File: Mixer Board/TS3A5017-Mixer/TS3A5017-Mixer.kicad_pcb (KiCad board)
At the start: 2 copper layers, 6 parts, among them J1 Conn_Coaxial_Small, J2 Conn_Coaxial_Small, J3 Conn_Coaxial_Small, U1 TS3A5017RGY, U2 LMP7715MF

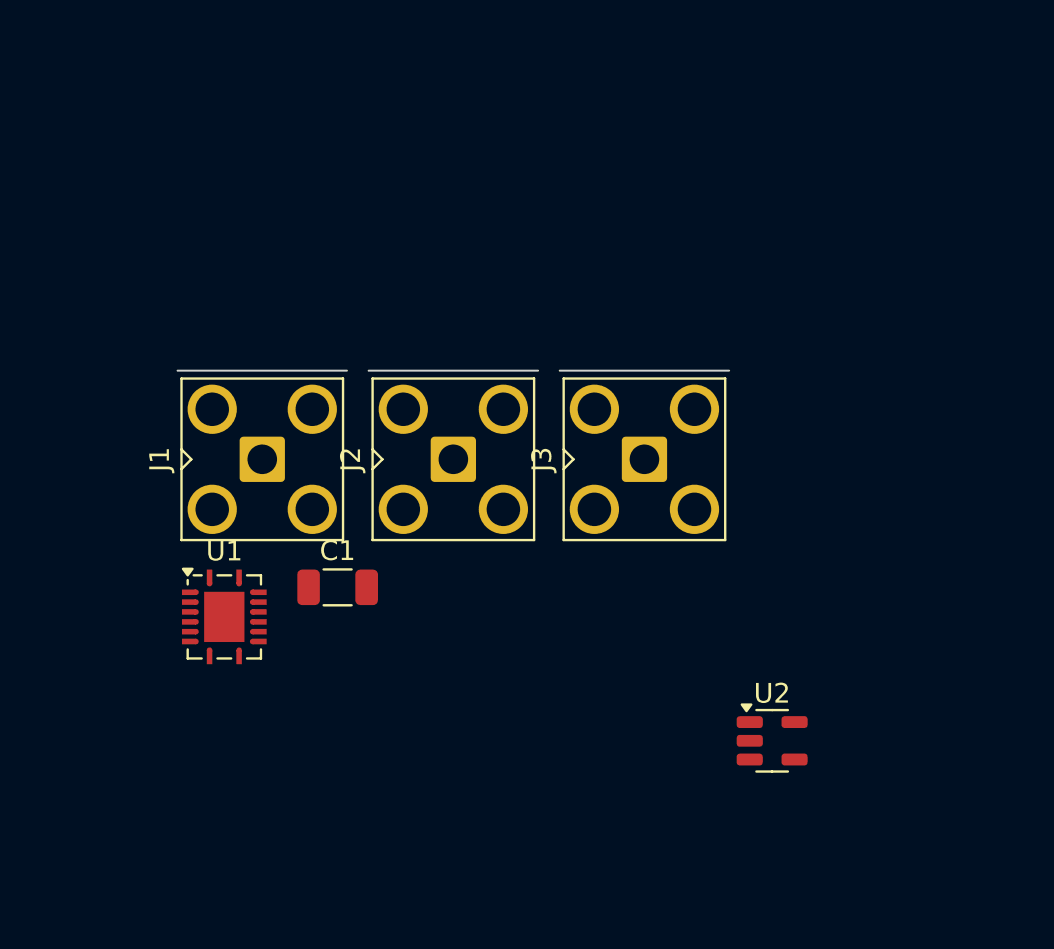
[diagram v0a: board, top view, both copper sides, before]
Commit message: Continued work and first iteration
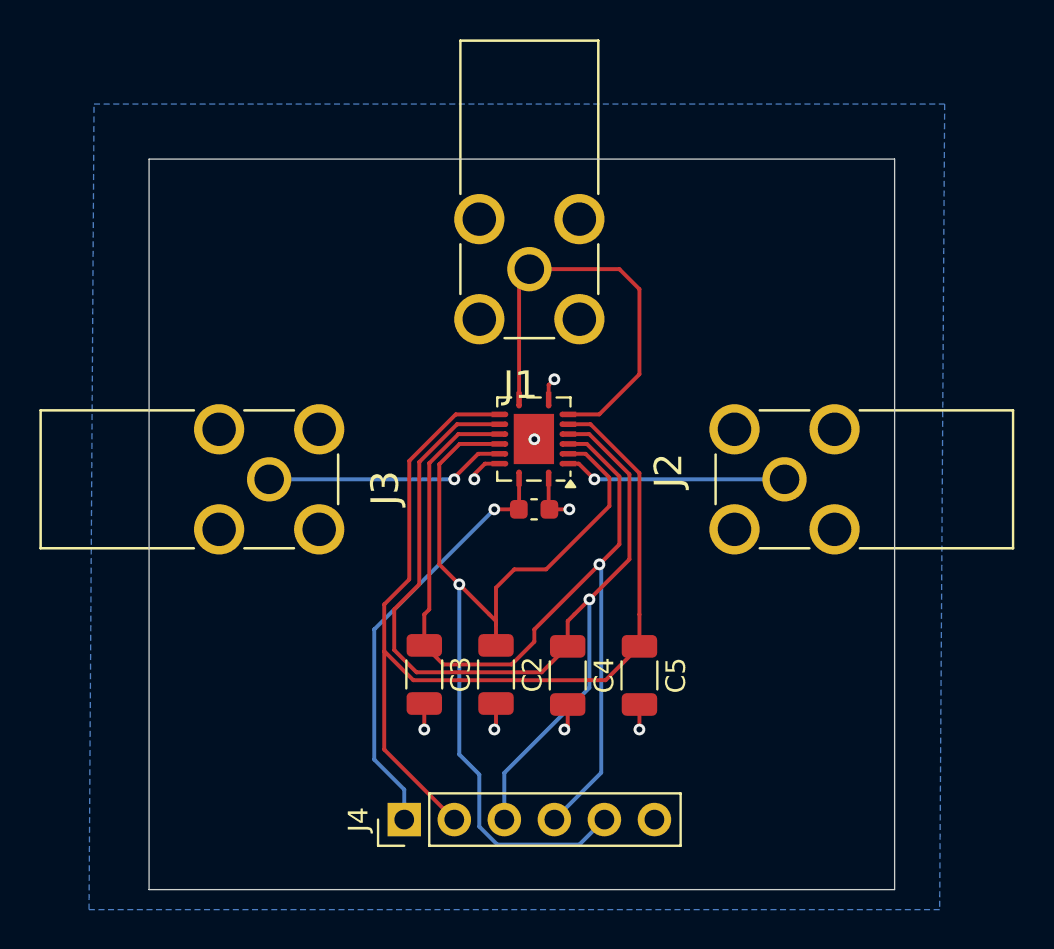
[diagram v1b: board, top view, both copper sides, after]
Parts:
- removed U2: LMP7715MF, Package_TO_SOT_SMD:SOT-23-5
- added C2: .1uf, Capacitor_SMD:C_1206_3216Metric, F.Cu at (144.9, 99.8)
- added C3: .1uf, Capacitor_SMD:C_1206_3216Metric, F.Cu at (141.2, 99.8)
- added C4: .1uf, Capacitor_SMD:C_1206_3216Metric, F.Cu at (148.5, 99.9)
- added C5: .1uf, Capacitor_SMD:C_1206_3216Metric, F.Cu at (152.1, 99.9)
- added J4: Conn_01x06, Connector_PinHeader_2.54mm:PinHeader_1x06_P2.54mm_Vertical, F.Cu at (140.2, 107.2)
- C1: footprint Capacitor_SMD:C_1206_3216Metric -> Capacitor_SMD:C_0603_1608Metric
- J1: value Conn_Coaxial_Small -> RF-In; footprint Connector_Coaxial:SMA_Amphenol_901-143_Horizontal -> Connector_Amphenol:AMPHENOL_901-143-6RFX
- J2: value Conn_Coaxial_Small -> CLK0; footprint Connector_Coaxial:SMA_Amphenol_901-143_Horizontal -> Connector_Amphenol:AMPHENOL_901-143-6RFX
- J3: value Conn_Coaxial_Small -> CLK1; footprint Connector_Coaxial:SMA_Amphenol_901-143_Horizontal -> Connector_Amphenol:AMPHENOL_901-143-6RFX
- moved J3 19.1 mm to (133.3, 89.9), turned to -90 degrees
- moved U1 18.1 mm to (146.8, 87.9), turned to 180 degrees
- moved J2 16.8 mm to (159.5, 89.9), turned to 90 degrees
- moved J1 16.6 mm to (146.6, 79.2), turned to 180 degrees
- moved C1 10.7 mm to (146.8, 91.4)
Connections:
- net Net-(U1-V+) renamed /3.3V
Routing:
- net Net-(J4-Pin_2): track 0.00 -> 53.5 mm
- net Net-(J4-Pin_3): track 0.00 -> 51.6 mm, vias 0 -> 1
- net Net-(J4-Pin_4): track 0.00 -> 47.3 mm, vias 0 -> 1
- net Net-(J4-Pin_5): track 0.00 -> 47.1 mm, vias 0 -> 1
- net /3.3V: track 0.00 -> 21.7 mm, vias 0 -> 1
- net RF-In: track 0.00 -> 21.5 mm
- net CLK1: track 0.00 -> 12.2 mm, vias 0 -> 1
- net CLK0: track 0.00 -> 11.3 mm, vias 0 -> 1
- net GND: track 0.00 -> 10.4 mm, vias 0 -> 8
- added copper zone on B.Cu, net GND
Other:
- board outline added: 37.8 x 37.1 mm
